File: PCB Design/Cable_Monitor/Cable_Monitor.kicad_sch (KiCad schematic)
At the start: 53 parts, among them J1 USB_B_Micro, P1 ${SIM.PARAMS}, P2 ${SIM.PARAMS}, Q1 BSS316N, SW1 On / Off Button, U1 SiP32508, U2 LD1117S33TR, U3 DRV5053_THT, U4 DRV5053_THT

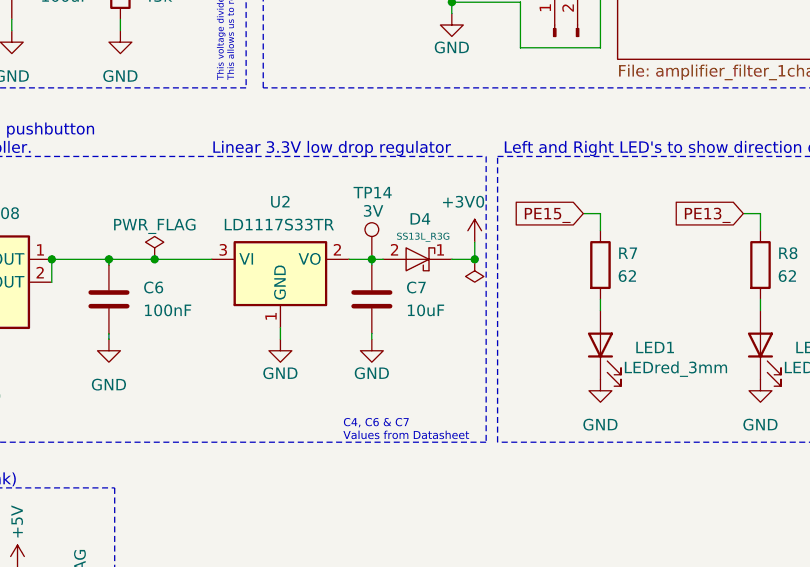
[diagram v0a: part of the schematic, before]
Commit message: Final Design Done
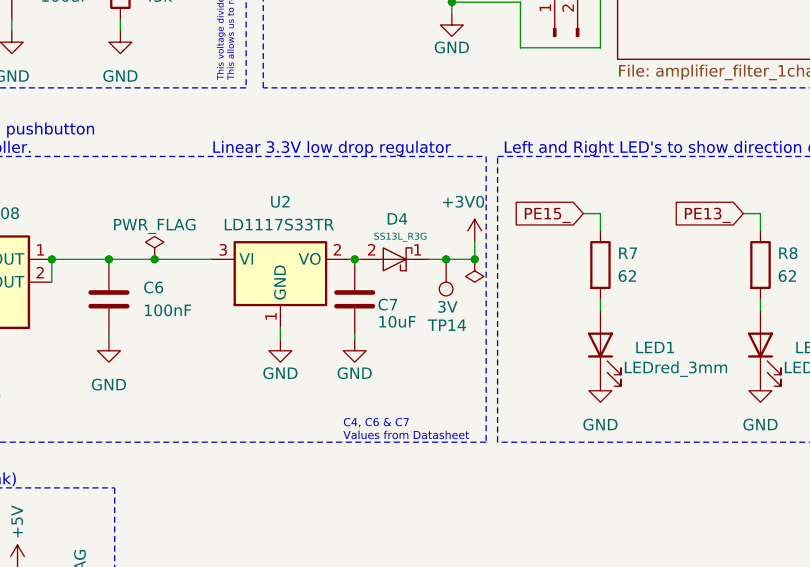
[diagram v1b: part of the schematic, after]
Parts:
- BZ1: footprint Buzzer_Beeper:Buzzer_12x9.5RM7.6 -> Buzzer_Beeper:Buzzer_D14mm_H7mm_P10mm
- J1: footprint Connector_USB:USB_Micro-B_Molex-105017-0001 -> Connector_USB:USB_Micro-B_Molex_47346-0001
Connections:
- net +3V0: now also TP14.1
- net at C7.1, D4.2 (A), U2.2 (VO): no longer TP14.1
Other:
- moved on the sheet: C7, D4, TP14
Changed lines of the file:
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@@
   (junction (at 217.805 87.63) (diameter 0) (color 0 0 0 0)
   )
+  (junction (at 205.74 127.635) (diameter 0) (color 0 0 0 0)
+  )
   (junction (at 220.345 49.53) (diameter 0) (color 0 0 0 0)
   )
@@
   (junction (at 88.265 92.075) (diameter 0) (color 0 0 0 0)
   )
+  (junction (at 195.58 127.635) (diameter 0) (color 0 0 0 0)
+  )
   (junction (at 206.375 38.1) (diameter 0) (color 0 0 0 0)
   )
@@
   )
   (junction (at 206.375 76.2) (diameter 0) (color 0 0 0 0)
-  )
-  (junction (at 197.485 127.635) (diameter 0) (color 0 0 0 0)
   )
   (junction (at 147.955 180.975) (diameter 0) (color 0 0 0 0)
@@
     (stroke (width 0) (type default))
   )
-  (wire (pts (xy 194.945 127.635) (xy 197.485 127.635))
+  (wire (pts (xy 194.945 127.635) (xy 195.58 127.635))
     (stroke (width 0) (type default))
   )
@@
     (stroke (width 0) (type default))
   )
-  (wire (pts (xy 197.485 127.635) (xy 198.755 127.635))
-    (stroke (width 0) (type default))
-  )
   (wire (pts (xy 216.535 87.63) (xy 217.805 87.63))
     (stroke (width 0) (type default))
@@
     (stroke (width 0) (type default))
   )
-  (wire (pts (xy 197.485 135.89) (xy 197.485 136.525))
+  (wire (pts (xy 195.58 135.89) (xy 195.58 136.525))
     (stroke (width 0) (type default))
   )
@@
     (stroke (width 0) (type default))
   )
-  (wire (pts (xy 206.375 127.635) (xy 208.915 127.635))
+  (wire (pts (xy 203.835 127.635) (xy 205.74 127.635))
     (stroke (width 0) (type default))
   )
@@
     (stroke (width 0) (type default))
   )
+  (wire (pts (xy 195.58 127.635) (xy 196.215 127.635))
+    (stroke (width 0) (type default))
+  )
   (wire (pts (xy 222.885 66.04) (xy 213.995 66.04))
     (stroke (width 0) (type default))
@@
     (stroke (width 0) (type default))
   )
+  (wire (pts (xy 205.74 127.635) (xy 208.915 127.635))
+    (stroke (width 0) (type default))
+  )
   (wire (pts (xy 54.61 125.73) (xy 46.99 125.73))
     (stroke (width 0) (type default))
@@
     (stroke (width 0) (type default))
   )
-  (wire (pts (xy 197.485 128.27) (xy 197.485 127.635))
+  (wire (pts (xy 195.58 128.27) (xy 195.58 127.635))
     (stroke (width 0) (type default))
   )
@@
     )
   )
-  (symbol (lib_id "power:GND") (at 197.485 136.525 0) (unit 1)
-    (in_bom yes) (on_board yes) (dnp no)
-    (property "Reference" "#PWR029" (at 197.485 142.875 0)
-      (effects (font (size 1.27 1.27)) hide)
-    )
-    (property "Value" "GND" (at 197.485 140.335 0)
-      (effects (font (size 1.27 1.27)))
-    )
-    (property "Footprint" "" (at 197.485 136.525 0)
-      (effects (font (size 1.27 1.27)) hide)
-    )
-    (property "Datasheet" "" (at 197.485 136.525 0)
+  (symbol (lib_id "power:GND") (at 195.58 136.525 0) (unit 1)
+    (in_bom yes) (on_board yes) (dnp no)
+    (property "Reference" "#PWR029" (at 195.58 142.875 0)
+      (effects (font (size 1.27 1.27)) hide)
+    )
+    (property "Value" "GND" (at 195.58 140.335 0)
+      (effects (font (size 1.27 1.27)))
+    )
+    (property "Footprint" "" (at 195.58 136.525 0)
+      (effects (font (size 1.27 1.27)) hide)
+    )
+    (property "Datasheet" "" (at 195.58 136.525 0)
       (effects (font (size 1.27 1.27)) hide)
     )
@@
     )
   )
-  (symbol (lib_id "Connector:TestPoint") (at 197.485 127.635 0) (unit 1)
-    (in_bom yes) (on_board yes) (dnp no)
-    (property "Reference" "TP14" (at 195.453 120.269 0)
-      (effects (font (size 1.27 1.27)) (justify left))
-    )
-    (property "Value" "3V" (at 196.469 122.301 0)
-      (effects (font (size 1.27 1.27)) (justify left))
-    )
-    (property "Footprint" "TestPoint:TestPoint_Loop_D2.60mm_Drill1.6mm_Beaded" (at 202.565 127.635 0)
-      (effects (font (size 1.27 1.27)) hide)
-    )
-    (property "Datasheet" "~" (at 202.565 127.635 0)
+  (symbol (lib_id "Connector:TestPoint") (at 205.74 127.635 0) (mirror x) (unit 1)
+    (in_bom yes) (on_board yes) (dnp no)
+    (property "Reference" "TP14" (at 203.708 135.001 0)
+      (effects (font (size 1.27 1.27)) (justify left))
+    )
+    (property "Value" "3V" (at 204.724 132.969 0)
+      (effects (font (size 1.27 1.27)) (justify left))
+    )
+    (property "Footprint" "TestPoint:TestPoint_Loop_D2.60mm_Drill1.6mm_Beaded" (at 210.82 127.635 0)
+      (effects (font (size 1.27 1.27)) hide)
+    )
+    (property "Datasheet" "~" (at 210.82 127.635 0)
       (effects (font (size 1.27 1.27)) hide)
     )
@@
       (effects (font (size 1.27 1.27)) (justify left))
     )
-    (property "Footprint" "Buzzer_Beeper:Buzzer_12x9.5RM7.6" (at 121.285 81.915 90)
-      (effects (font (size 1.27 1.27)) hide)
-    )
-    (property "Datasheet" "~" (at 121.285 81.915 90)
+    (property "Footprint" "Buzzer_Beeper:Buzzer_D14mm_H7mm_P10mm" (at 121.285 81.915 90)
+      (effects (font (size 1.27 1.27)) hide)
+    )
+    (property "Datasheet" "https://media.distrelec.com/Web/Downloads/_t/ds/RND%20430-00017_eng_tds.pdf" (at 121.285 81.915 90)
       (effects (font (size 1.27 1.27)) hide)
     )
@@
     )
   )
-  (symbol (lib_id "Device:C") (at 197.485 132.08 0) (unit 1)
-    (in_bom yes) (on_board yes) (dnp no) (fields_autoplaced)
-    (property "Reference" "C7" (at 201.295 130.8099 0)
-      (effects (font (size 1.27 1.27)) (justify left))
-    )
-    (property "Value" "10uF" (at 201.295 133.3499 0)
-      (effects (font (size 1.27 1.27)) (justify left))
-    )
-    (property "Footprint" "Capacitor_SMD:C_0805_2012Metric_Pad1.18x1.45mm_HandSolder" (at 198.4502 135.89 0)
-      (effects (font (size 1.27 1.27)) hide)
-    )
-    (property "Datasheet" "~" (at 197.485 132.08 0)
+  (symbol (lib_id "Device:C") (at 195.58 132.08 0) (unit 1)
+    (in_bom yes) (on_board yes) (dnp no)
+    (property "Reference" "C7" (at 198.12 132.715 0)
+      (effects (font (size 1.27 1.27)) (justify left))
+    )
+    (property "Value" "10uF" (at 198.12 134.62 0)
+      (effects (font (size 1.27 1.27)) (justify left))
+    )
+    (property "Footprint" "Capacitor_SMD:C_0805_2012Metric_Pad1.18x1.45mm_HandSolder" (at 196.5452 135.89 0)
+      (effects (font (size 1.27 1.27)) hide)
+    )
+    (property "Datasheet" "~" (at 195.58 132.08 0)
       (effects (font (size 1.27 1.27)) hide)
     )
@@
     )
   )
-  (symbol (lib_id "SS13L_R3G:SS13L_R3G") (at 206.375 127.635 180) (unit 1)
-    (in_bom yes) (on_board yes) (dnp no)
-    (property "Reference" "D4" (at 202.8444 123.19 0)
-      (effects (font (size 1.27 1.27)))
-    )
-    (property "Value" "SS13L_R3G" (at 203.2 125.095 0)
+  (symbol (lib_id "SS13L_R3G:SS13L_R3G") (at 203.835 127.635 180) (unit 1)
+    (in_bom yes) (on_board yes) (dnp no)
+    (property "Reference" "D4" (at 200.3044 123.19 0)
+      (effects (font (size 1.27 1.27)))
+    )
+    (property "Value" "SS13L_R3G" (at 200.66 125.095 0)
       (effects (font (size 0.762 0.762)))
     )
-    (property "Footprint" "SS13L_R3G:SODFL3618X143N" (at 197.485 30.175 0)
+    (property "Footprint" "SS13L_R3G:SODFL3618X143N" (at 194.945 30.175 0)
       (effects (font (size 1.27 1.27)) (justify left top) hide)
     )
-    (property "Datasheet" "https://www.arrow.com/en/products/ss13l-r3g/taiwan-semiconductor" (at 197.485 -69.825 0)
+    (property "Datasheet" "https://www.arrow.com/en/products/ss13l-r3g/taiwan-semiconductor" (at 194.945 -69.825 0)
       (effects (font (size 1.27 1.27)) (justify left top) hide)
     )
-    (property "Height" "1.43" (at 197.485 -269.825 0)
+    (property "Height" "1.43" (at 194.945 -269.825 0)
       (effects (font (size 1.27 1.27)) (justify left top) hide)
     )
-    (property "Manufacturer_Name" "Taiwan Semiconductor" (at 197.485 -369.825 0)
+    (property "Manufacturer_Name" "Taiwan Semiconductor" (at 194.945 -369.825 0)
       (effects (font (size 1.27 1.27)) (justify left top) hide)
     )
-    (property "Manufacturer_Part_Number" "SS13L R3G" (at 197.485 -469.825 0)
+    (property "Manufacturer_Part_Number" "SS13L R3G" (at 194.945 -469.825 0)
       (effects (font (size 1.27 1.27)) (justify left top) hide)
     )
-    (property "Mouser Part Number" "821-SS13LR3G" (at 197.485 -569.825 0)
+    (property "Mouser Part Number" "821-SS13LR3G" (at 194.945 -569.825 0)
       (effects (font (size 1.27 1.27)) (justify left top) hide)
     )
-    (property "Mouser Price/Stock" "https://www.mouser.co.uk/ProductDetail/Taiwan-Semiconductor/SS13L-R3G?qs=5aG0NVq1C4yK%252B2Aj4Chtgw%3D%3D" (at 197.485 -669.825 0)
+    (property "Mouser Price/Stock" "https://www.mouser.co.uk/ProductDetail/Taiwan-Semiconductor/SS13L-R3G?qs=5aG0NVq1C4yK%252B2Aj4Chtgw%3D%3D" (at 194.945 -669.825 0)
       (effects (font (size 1.27 1.27)) (justify left top) hide)
     )
-    (property "Arrow Part Number" "SS13L R3G" (at 197.485 -769.825 0)
+    (property "Arrow Part Number" "SS13L R3G" (at 194.945 -769.825 0)
       (effects (font (size 1.27 1.27)) (justify left top) hide)
     )
-    (property "Arrow Price/Stock" "https://www.arrow.com/en/products/ss13l-r3g/taiwan-semiconductor" (at 197.485 -869.825 0)
+    (property "Arrow Price/Stock" "https://www.arrow.com/en/products/ss13l-r3g/taiwan-semiconductor" (at 194.945 -869.825 0)
       (effects (font (size 1.27 1.27)) (justify left top) hide)
     )
@@
       (effects (font (size 1.27 1.27)))
     )
-    (property "Footprint" "Connector_USB:USB_Micro-B_Molex-105017-0001" (at 144.145 170.815 0)
-      (effects (font (size 1.27 1.27)) hide)
-    )
+    (property "Footprint" "Connector_USB:USB_Micro-B_Molex_47346-0001" (at 144.145 170.815 0)
+      (effects (font (size 1.27 1.27)) hide)
+    )
